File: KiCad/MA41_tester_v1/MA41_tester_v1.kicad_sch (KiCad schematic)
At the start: 5 parts

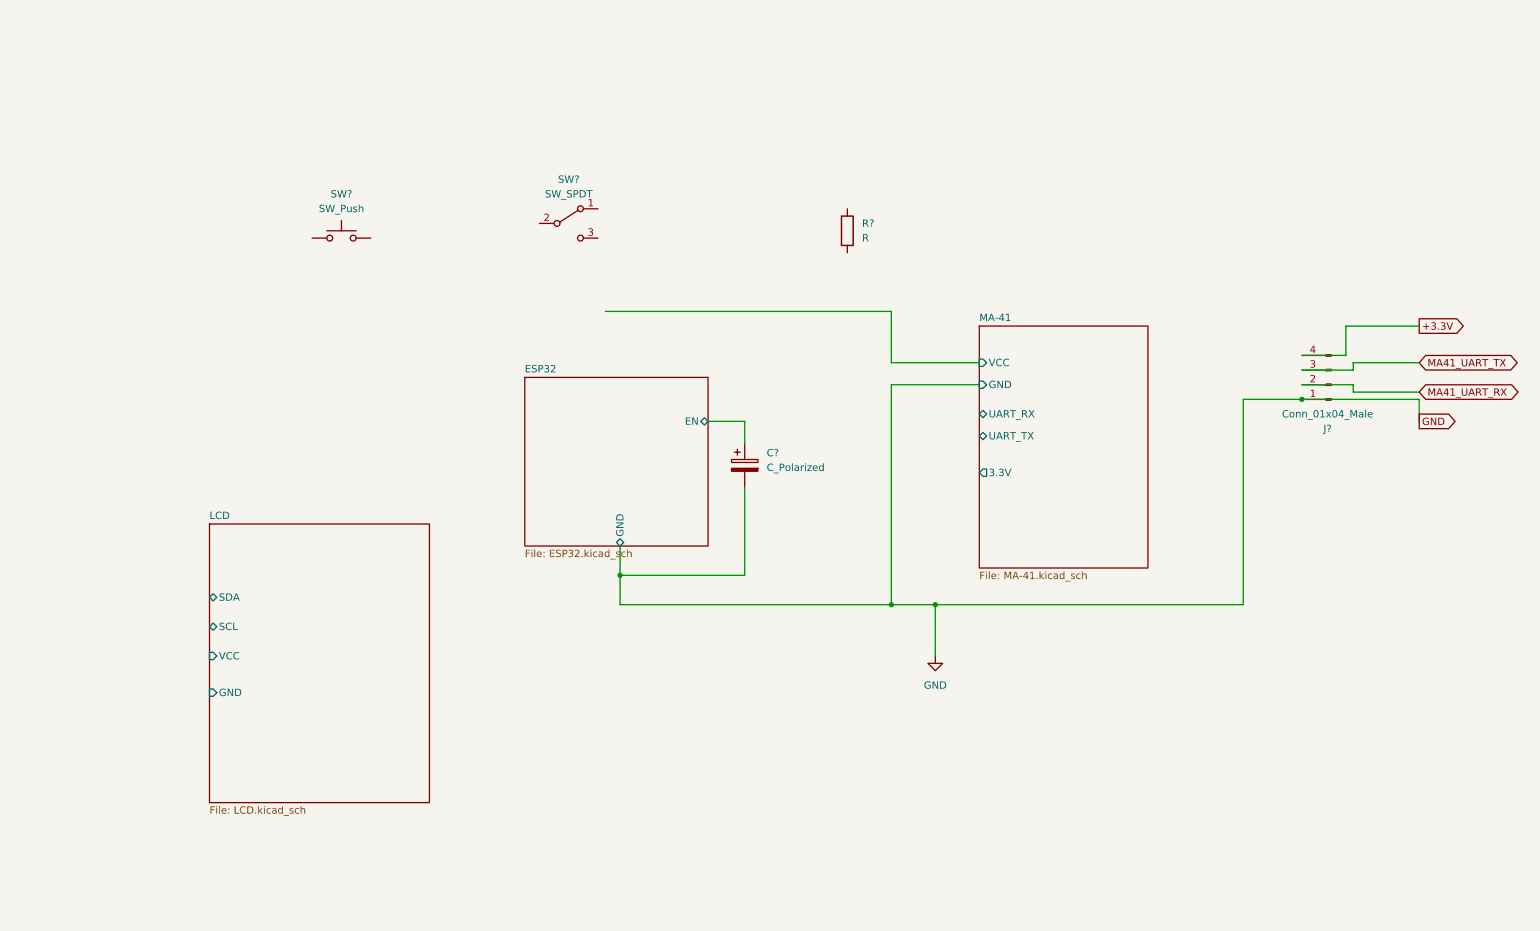
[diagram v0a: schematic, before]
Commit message: ююю
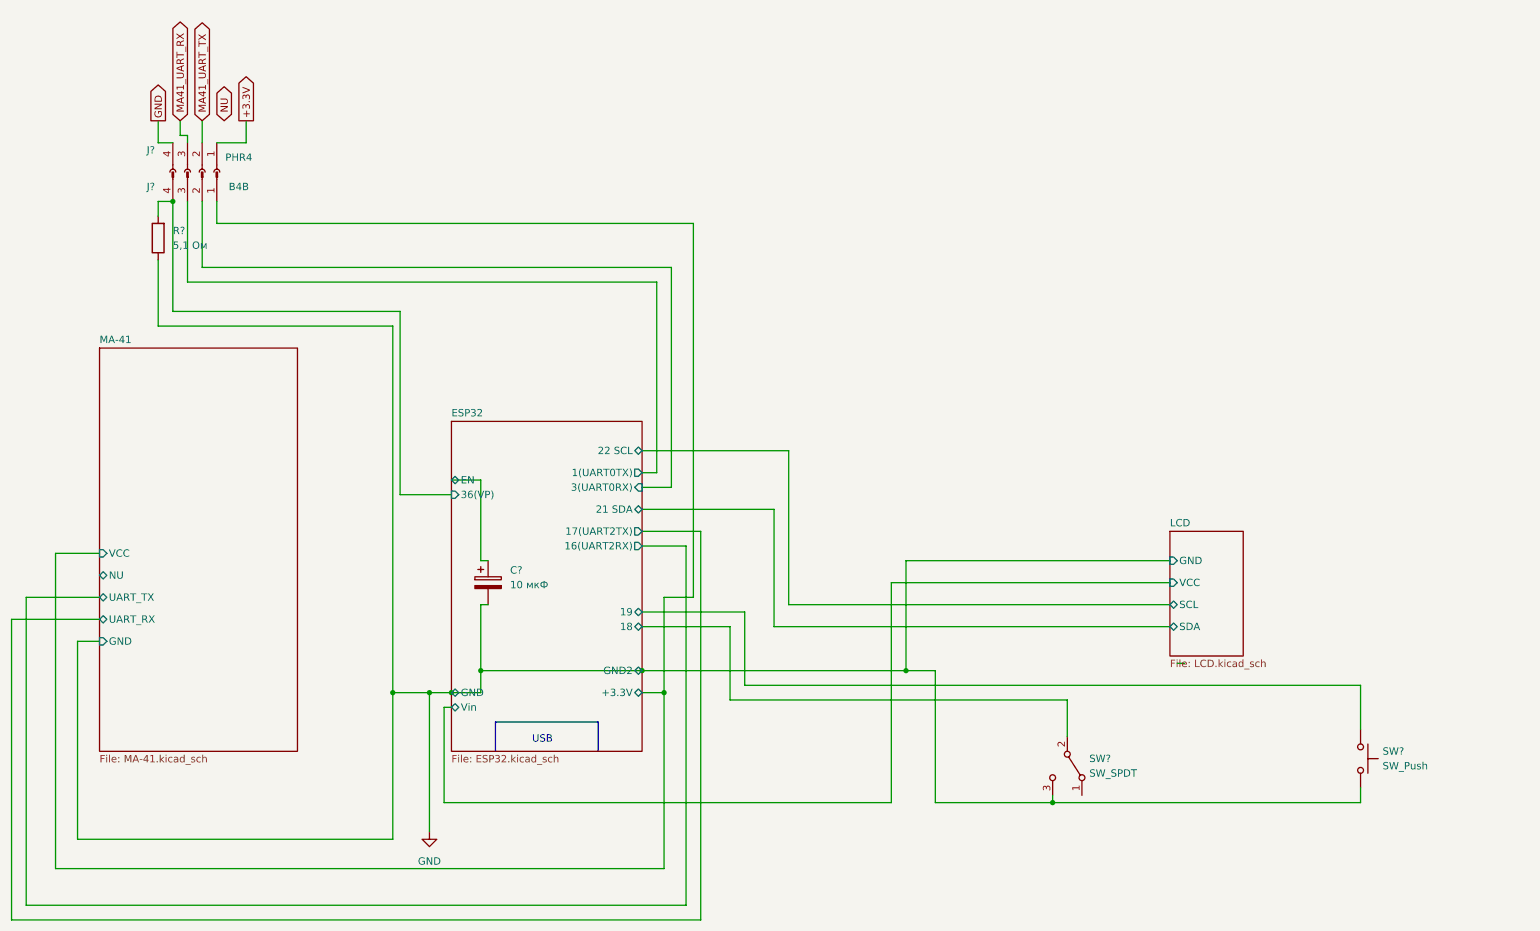
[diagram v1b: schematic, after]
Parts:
- added J?: PHR4, symbol Connector:Conn_01x04_Female
- C?: value C_Polarized -> 10 мкФ
- J?: value Conn_01x04_Male -> B4B
- R?: value R -> 5,1 Ом
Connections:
- net +3.3V: now also J?.1 (Pin_1); no longer J?.4 (Pin_4)
- net GND: now also R?.1, SW?.2, SW?.3 (C), J?.4 (Pin_4); no longer J?.1 (Pin_1)
- net MA41_UART_RX: now also J?.3 (Pin_3); no longer J?.2 (Pin_2)
- net MA41_UART_TX: now also J?.2 (Pin_2); no longer J?.3 (Pin_3)
- net ESP32/18: now reaches SW?.2 (B)
- net ESP32/36(VP): now reaches R?.2
- net ESP32/36(VP): now also J?.4 (Pin_4)
- net ESP32/19: now reaches SW?.1
- new net ESP32/+3.3V: J?.1 (Pin_1)
- new net ESP32/1(UART0TX): J?.3 (Pin_3)
- new net ESP32/3(UART0RX): J?.2 (Pin_2)
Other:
- sheet ESP32 ports: added +3.3V, 1(UART0TX), 16(UART2RX), 17(UART2TX), 18, 19, 21 SDA, 22 SCL, 3(UART0RX), 36(VP), GND2, Vin; removed none
- sheet MA-41 ports: added NU; removed 3.3V
- note added: "USB"
- moved on the sheet: C?, J?, R?, SW?
